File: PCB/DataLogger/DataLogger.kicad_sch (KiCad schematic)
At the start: 19 parts, among them J1 Power, U2 DS18B20, U3 DS18B20, U4 DS18B20, U5 SHT30-DIS

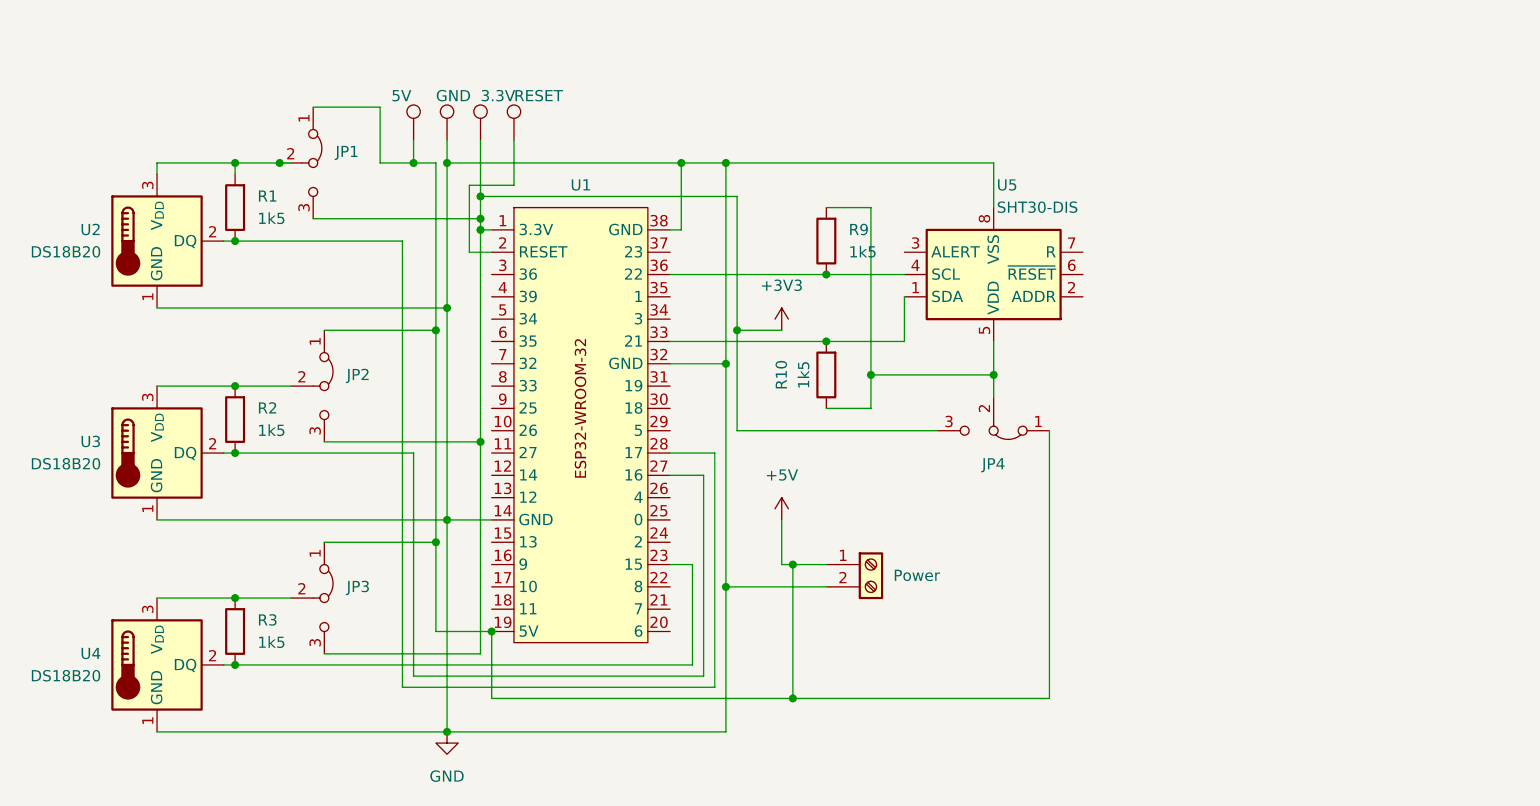
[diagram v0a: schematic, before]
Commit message: Ordered Board
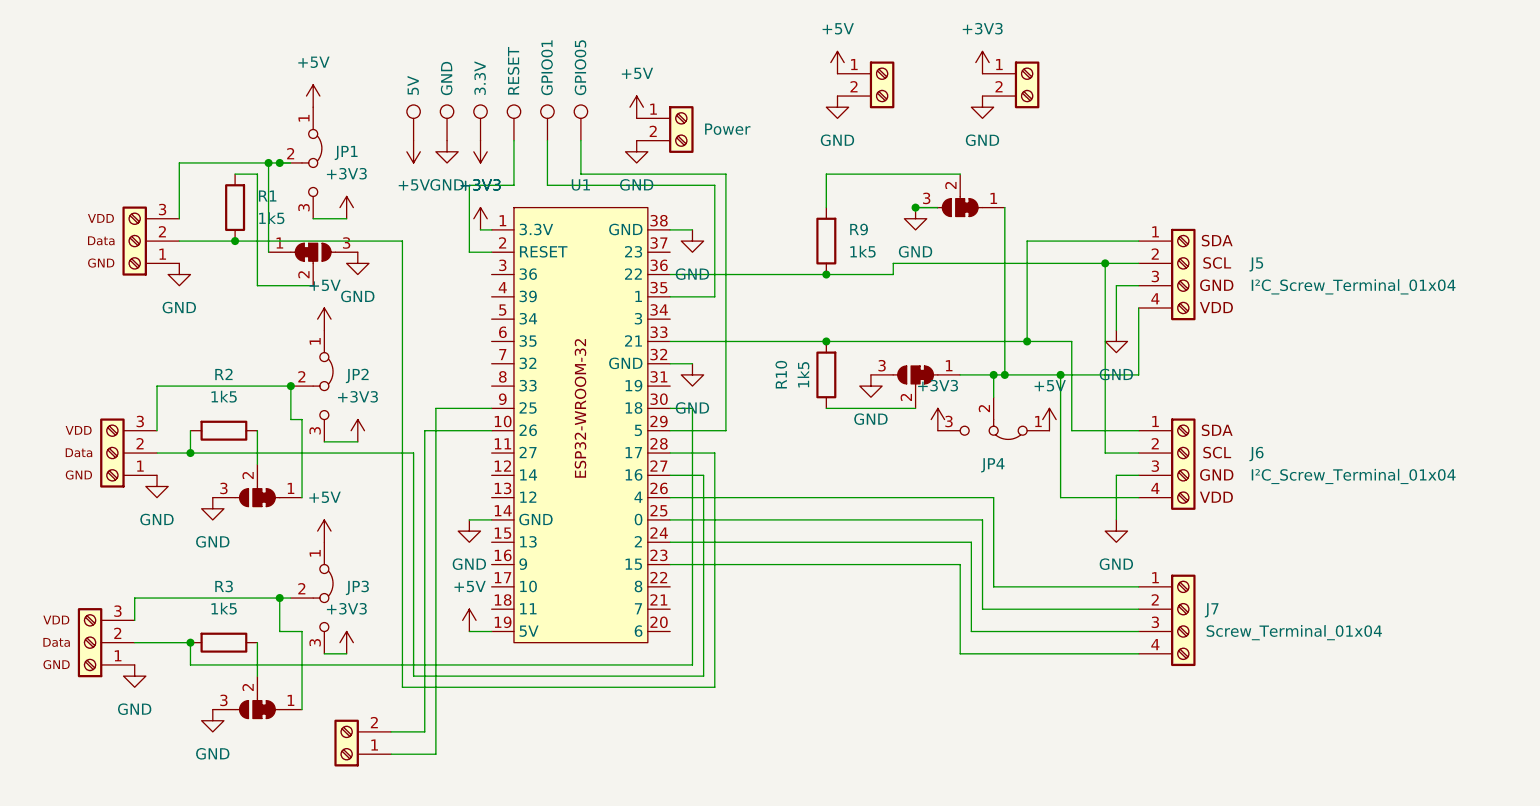
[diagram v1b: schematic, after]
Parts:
- removed U2, U3, U4: DS18B20, ESP32Board:Screw Terminal 3*2.54 1WI, symbol Sensor_Temperature:DS18B20
- removed U5: SHT30-DIS, ESP32Board:Screw Terminal 4*2.54 SHT30, symbol Sensor_Humidity:SHT30-DIS
- added J10, J8, J9: Screw_Terminal_01x02, ESP32Board:Screw Terminal 2*2.54, symbol Connector:Screw_Terminal_01x02
- added J2, J3, J4: 1WI Screw_Terminal_01x03, ESP32Board:Screw Terminal 3*2.54 1WI, symbol ESP32Board:1WI Screw_Terminal_01x03
- added J5, J6: I²C_Screw_Terminal_01x04, ESP32Board:Screw Terminal 4*2.54 I²C, symbol ESP32Board:I²C_Screw_Terminal_01x04
- added J7: Screw_Terminal_01x04, ESP32Board:Screw Terminal 4*2.54, symbol Connector:Screw_Terminal_01x04
- added JP5, JP6, JP7, JP8, JP9: SolderJumper_3_Bridged12, Jumper:SolderJumper-3_P1.3mm_Bridged12_RoundedPad1.0x1.5mm_NumberLabels, symbol Jumper:SolderJumper_3_Bridged12
- added TP5: GPIO01, TestPoint:TestPoint_THTPad_D1.5mm_Drill0.7mm, symbol Connector:TestPoint
- added TP6: GPIO05, TestPoint:TestPoint_THTPad_D1.5mm_Drill0.7mm, symbol Connector:TestPoint
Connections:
- net +3V3: now also J9.1 (Pin_1)
- net +5V: now also J8.1 (Pin_1)
- net GND: now also J2.1 (GND), J3.1 (GND), J4.1 (GND), J5.3 (GND), J6.3 (GND), J8.2 (Pin_2), J9.2 (Pin_2), JP5.3 (B), JP6.3 (B), JP7.3 (B), JP8.3 (B), JP9.3 (B)
- net at R2.1: now also JP6.2 (C); no longer U1.27 (16)
- net at JP2.2 (C): now also J3.3 (VDD), JP6.1 (A); no longer R2.2
- net at JP1.2 (C): now also J2.3 (VDD), JP5.1 (A); no longer R1.2
- net at R9.1, U1.36 (22): now also J5.2 (SCL), J6.2 (SCL)
- net at R3.1: now also JP7.2 (C); no longer U1.23 (15)
- net at R3.2: now also U1.30 (18), J4.2 (Data); no longer JP3.2 (C)
- net at R1.1, U1.28 (17): now also J2.2 (Data)
- net at R10.2, U1.33 (21): now also J5.1 (SDA), J6.1 (SDA)
- net at U1.10 (26): now also J10.2 (Pin_2)
- net at U1.24 (2): now also J7.3 (Pin_3)
- net at U1.25 (0): now also J7.2 (Pin_2)
- net at U1.26 (4): now also J7.1 (Pin_1)
- net at U1.29 (5): now also TP6.1
- net at U1.35 (1): now also TP5.1
- net at U1.9 (25): now also J10.1 (Pin_1)
- new net: J4.3 (VDD), JP3.2 (C), JP7.1 (A)
- new net: J5.4 (VDD), J6.4 (VDD), JP4.2 (C), JP8.1 (A), JP9.1 (A)
- new net: JP9.2 (C), R10.1
- new net: JP5.2 (C), R1.2
- new net: JP8.2 (C), R9.2
- new net: J3.2 (Data), R2.2, U1.27 (16)
- new net: J7.4 (Pin_4), U1.23 (15)
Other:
- moved on the sheet: R2, R3
